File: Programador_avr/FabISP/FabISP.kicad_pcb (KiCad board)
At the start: 2 copper layers, 31.5 x 59.5 mm, 14 parts, among them IC1 ATTINY44-SSU, M1 RESONATOR, M2 PINHD-1x02-SMD-HEADER, M3 MICRO-USB_1_64

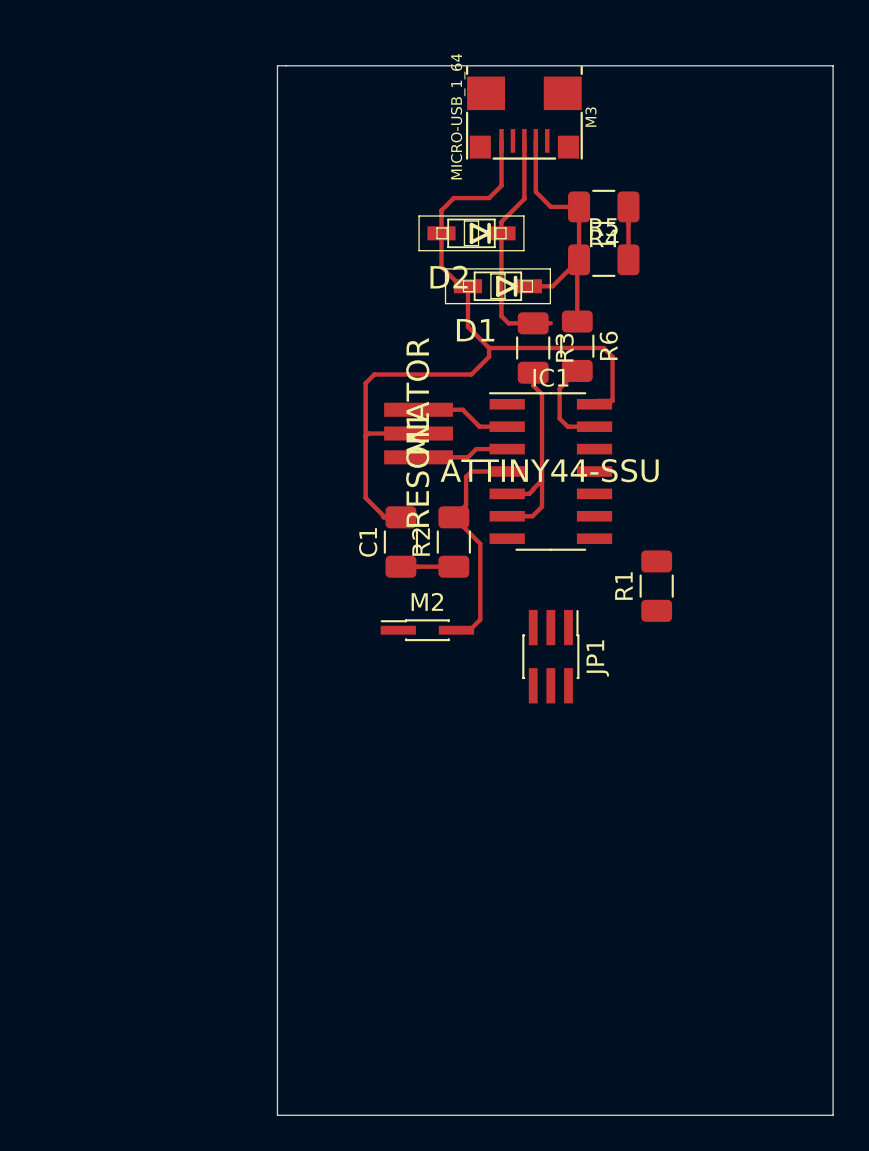
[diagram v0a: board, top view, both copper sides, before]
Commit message: pcb 90%
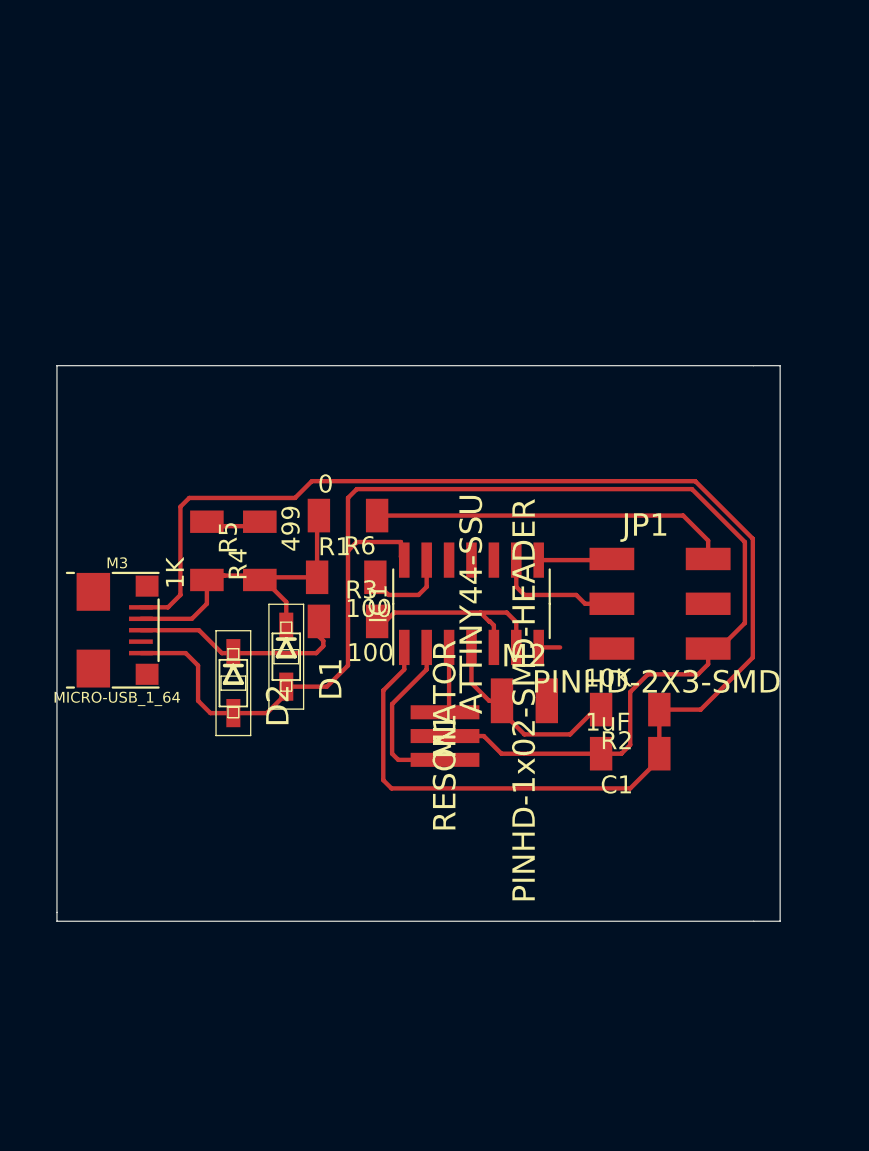
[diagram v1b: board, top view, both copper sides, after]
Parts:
- C1: footprint Capacitor_SMD:C_1206_3216Metric -> fab:fab-C1206FAB
- JP1: footprint Connector_PinHeader_1.00mm:PinHeader_2x03_P1.00mm_Vertical_SMD -> fab:fab-2X03SMD
- M2: footprint Connector_PinHeader_1.00mm:PinHeader_2x01_P1.00mm_Vertical_SMD -> fab:fab-1X02SMD
- R1, R2, R3, R4, R5, R6: footprint Resistor_SMD:R_1206_3216Metric -> fab:fab-R1206FAB
- moved M3 37.5 mm to (74.7, 61.5), turned to 270 degrees
- moved R4 29.8 mm to (80.0, 57.0), turned to 270 degrees
- moved D2 28.9 mm to (81.5, 64.5), turned to 270 degrees
- moved R5 25.5 mm to (83.0, 57.0), turned to 90 degrees
- moved D1 24.2 mm to (84.5, 63.0), turned to 270 degrees
- moved R3 18.7 mm to (88.0, 61.0), turned to 0 degrees
- moved R6 18.5 mm to (87.9, 58.5), turned to 0 degrees
- moved R1 18.0 mm to (88.0, 55.0), turned to 180 degrees
- moved C1 17.7 mm to (104.0, 68.5), turned to 180 degrees
- moved M1 17.2 mm to (93.5, 67.5), turned to 90 degrees
- moved R2 13.8 mm to (104.0, 66.0), turned to 180 degrees
- moved IC1 8.75 mm to (95.0, 60.0), turned to 90 degrees
- moved M2 6.80 mm to (98.0, 65.5), turned to 270 degrees
- moved JP1 6.71 mm to (105.5, 60.0), turned to 0 degrees
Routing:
- net VCC: track 3.00 -> 82.6 mm
- net GND: track 46.7 -> 80.8 mm
- net Net-(JP1-Pad2): track 0.00 -> 20.4 mm
- net /SCK: track 0.00 -> 7.33 mm
- net /XTAL1: track 5.42 -> 9.98 mm
- net /MISO: track 0.00 -> 4.18 mm
- net /D-: track 15.8 -> 19.3 mm
- net /PB3: track 13.1 -> 11.5 mm
- net /XTAL2: track 5.22 -> 3.77 mm
- net /MOSI: track 0.00 -> 1.22 mm
- net /D+: track 13.4 -> 12.5 mm
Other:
- board size 31.5 x 59.5 mm -> 41 x 31.5 mm
